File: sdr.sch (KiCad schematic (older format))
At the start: 3 parts

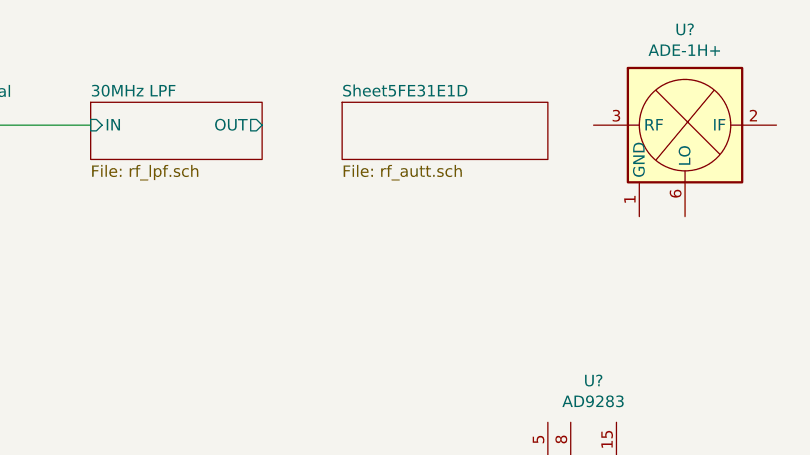
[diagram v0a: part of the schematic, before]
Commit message: Attenuator revised
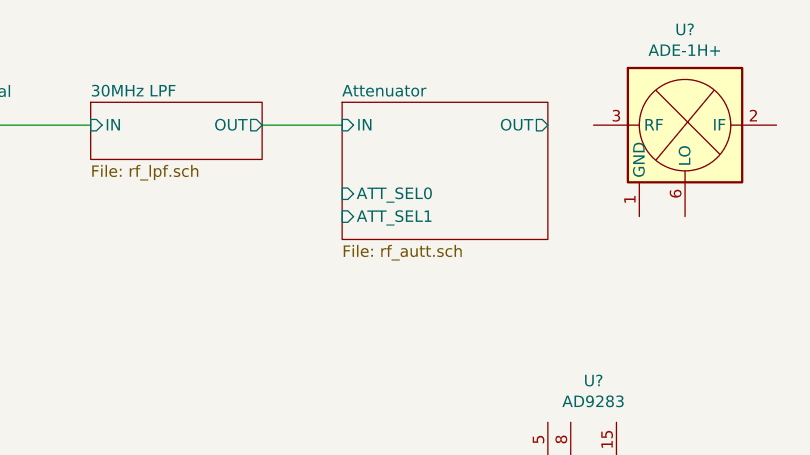
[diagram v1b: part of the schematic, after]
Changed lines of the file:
@@
 F3 "OUT" O R 2250 3450 50
-$EndSheet
-$Sheet
-S 2600 3350 900  250
-U 5FE31E1E
-F0 "Sheet5FE31E1D" 50
-F1 "rf_autt.sch" 50
 $EndSheet
 $Comp
@@
 	1    0    0    -1
 $EndComp
+$Sheet
+S 2600 3350 900  600
+U 5FE31E1E
+F0 "Attenuator" 50
+F1 "rf_autt.sch" 50
+F2 "IN" I L 2600 3450 50
+F3 "OUT" O R 3500 3450 50
+F4 "ATT_SEL0" I L 2600 3750 50
+F5 "ATT_SEL1" I L 2600 3850 50
+$EndSheet
+Wire Wire Line
+	2250 3450 2600 3450
 $EndSCHEMATC
